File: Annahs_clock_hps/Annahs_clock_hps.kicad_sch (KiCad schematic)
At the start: 4 parts

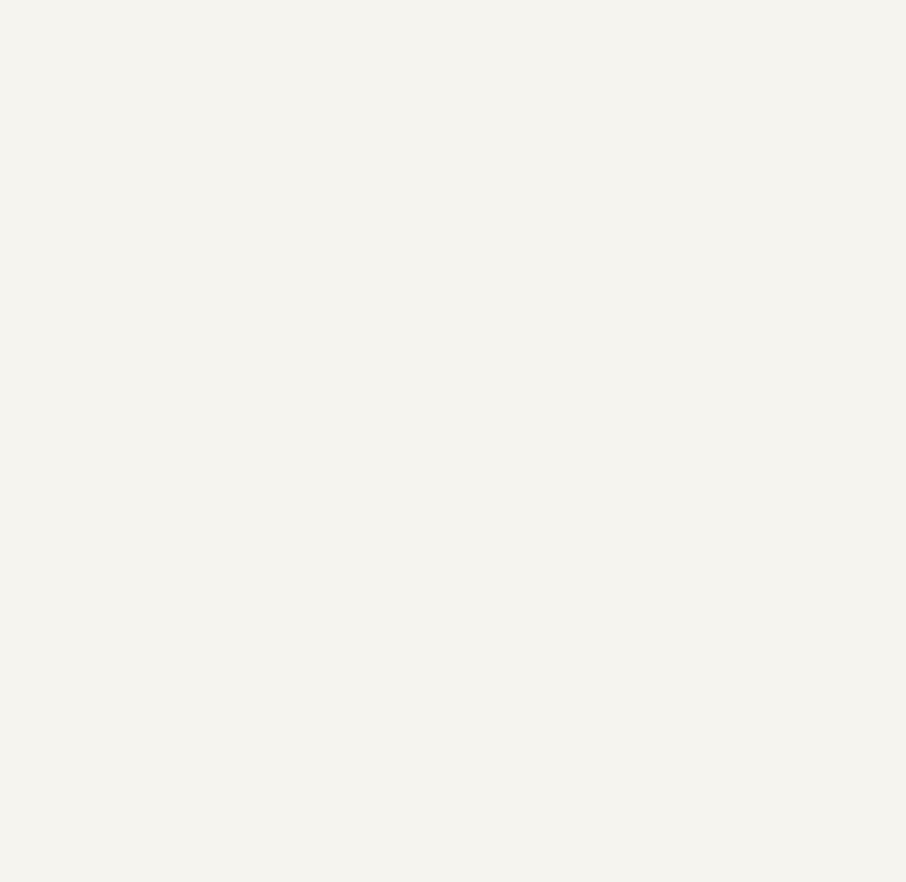
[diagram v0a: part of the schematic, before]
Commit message: Slide 39
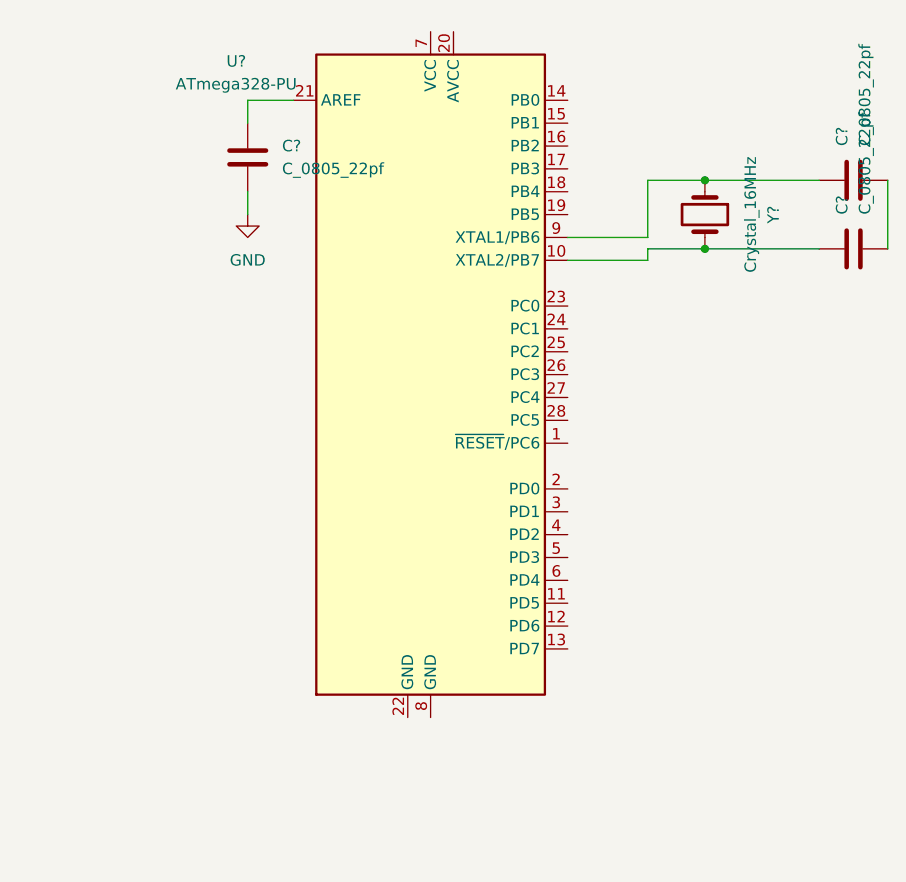
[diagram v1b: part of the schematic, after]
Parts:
- added C? (x3): C_0805_22pf, footprints:C_0805_2012Metric, symbol HPS:C_0805_22pf
- added U?: ATmega328-PU, footprints:DIP-28_W7.62mm, symbol HPS:ATmega328-PU
- added Y?: Crystal_16MHz, footprints:Crystal_SMD_HC49-SD, symbol HPS:Crystal_16MHz
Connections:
- new net: C?.1, U?.9 (XTAL1/PB6), Y?.1
- new net: C?.2, C?.2
- new net: C?.1, U?.10 (XTAL2/PB7), Y?.2
- new net: C?.1, U?.21 (AREF)
- new net GND: C?.2
